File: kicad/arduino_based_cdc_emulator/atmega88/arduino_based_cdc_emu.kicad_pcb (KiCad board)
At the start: 2 copper layers, 13 parts, among them IC1 ATMEGA88-A, P1 CONN_5, P2 CONN_2, U1 78L05, X1 20MHz

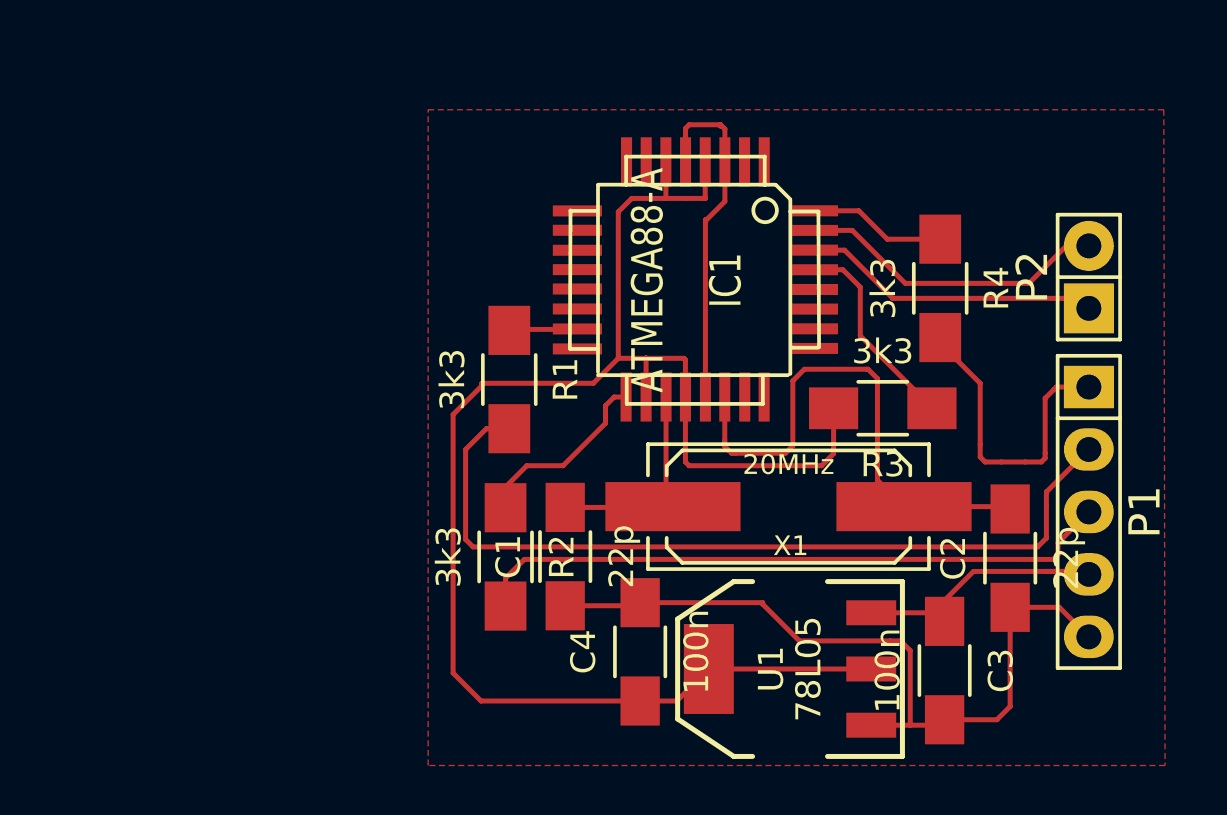
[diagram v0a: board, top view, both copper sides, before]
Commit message: same changes
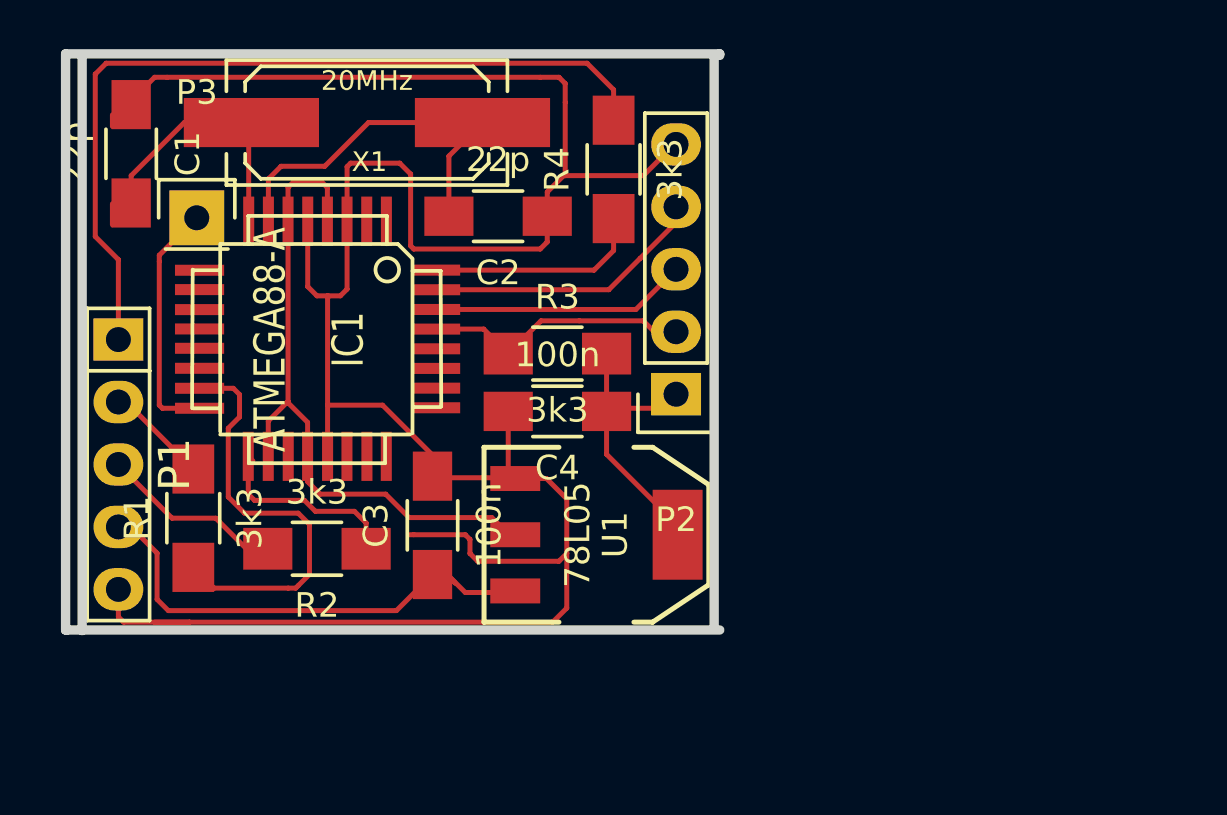
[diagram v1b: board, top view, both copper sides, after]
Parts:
- added P3: CONN_3, Pin_Headers:Pin_Header_Straight_1x01, F.Cu at (104.6, 107.1)
- P1: value CONN_5 -> CONN_1
- P2: footprint Pin_Headers:Pin_Header_Straight_1x02 -> Pin_Headers:Pin_Header_Straight_1x05
- moved P1 39.5 mm to (101.4, 117.1)
- moved C2 25.0 mm to (116.8, 107.0), turned to 180 degrees
- moved C1 24.1 mm to (101.9, 104.5), turned to 270 degrees
- moved X1 23.2 mm to (111.5, 103.2)
- moved C3 21.6 mm to (114.2, 119.6), turned to 90 degrees
- moved P2 17.5 mm to (124.1, 114.2), turned to 180 degrees
- moved IC1 15.6 mm to (109.5, 112.0)
- moved R4 14.1 mm to (121.5, 105.1), turned to 90 degrees
- moved R1 14.0 mm to (104.4, 119.3), turned to 90 degrees
- moved R3 13.4 mm to (119.3, 112.6), turned to 0 degrees
- moved C4 10.3 mm to (119.3, 114.9), turned to 180 degrees
- moved U1 9.58 mm to (120.8, 120.0), turned to 270 degrees
- moved R2 7.68 mm to (109.5, 120.5), turned to 180 degrees
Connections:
- IC1 pad 16: (no net) -> /MISO
- IC1 pad 19: Net-(C1-Pad2) -> (no net)
- IC1 pad 22: Net-(C2-Pad2) -> (no net)
- IC1 pad 29: Net-(IC1-Pad29) -> /RESET
- IC1 pad 7: (no net) -> Net-(C2-Pad2)
- IC1 pad 8: (no net) -> Net-(C1-Pad2)
- P2 pad 1: RX -> +5V
- P2 pad 2: TX -> /RESET
- R3 pad 1: Net-(IC1-Pad29) -> /RESET
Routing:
- net GND: track 46.7 -> 106.8 mm
- net /DataIn: track 34.0 -> 4.40 mm
- net +5V: track 65.6 -> 40.8 mm
- net /DataOut: track 12.7 -> 34.1 mm
- net /Clock: track 26.3 -> 7.78 mm
- net Net-(IC1-Pad15): track 3.04 -> 17.2 mm
- net /RESET: track 0.00 -> 11.9 mm
- net /MISO: track 0.00 -> 9.94 mm
- net +12V: track 10.8 -> 20.1 mm
- net Net-(IC1-Pad29): track 8.33 -> 0.00 mm
- net Net-(C2-Pad2): track 23.4 -> 17.5 mm
- net Net-(C1-Pad2): track 10.2 -> 14.8 mm
- net Net-(IC1-Pad32): track 5.63 -> 8.87 mm
- net RX: track 12.2 -> 10.5 mm
- net TX: track 12.7 -> 11.5 mm
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- removed copper zone on F.Cu, net GND
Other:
- board outline added: 26.6 x 23.5 mm
